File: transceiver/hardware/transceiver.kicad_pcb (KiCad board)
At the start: 2 copper layers, 50 x 50 mm, 62 parts, among them J1 Conn_Coaxial, J2 Conn_Coaxial, J3 Conn_01x04, J4 Conn_01x02, J5 Conn_Coaxial, U2 LR2021, U3 STM32G030K8Tx, U4 MAX-M10S, Y1 32.768KHz, Y3 32MHz 10pF

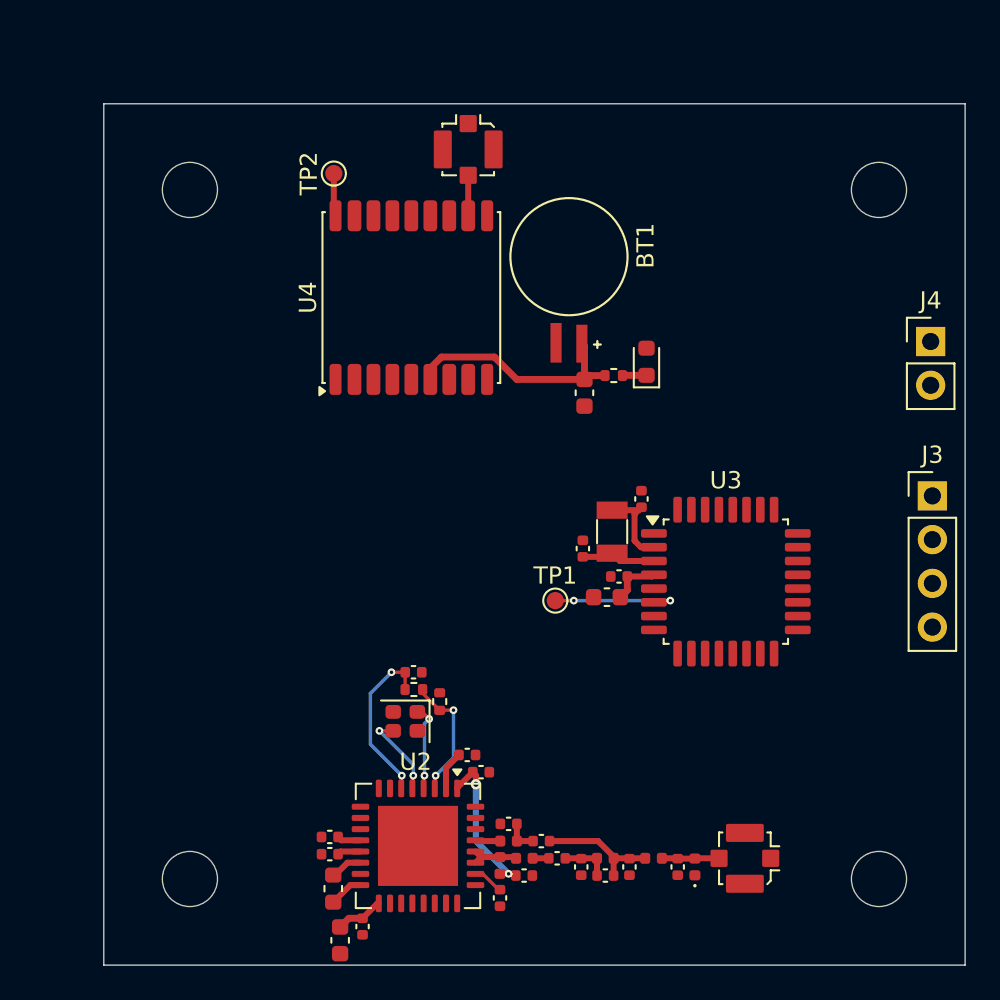
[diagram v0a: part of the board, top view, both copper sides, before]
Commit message: updated board and started frame
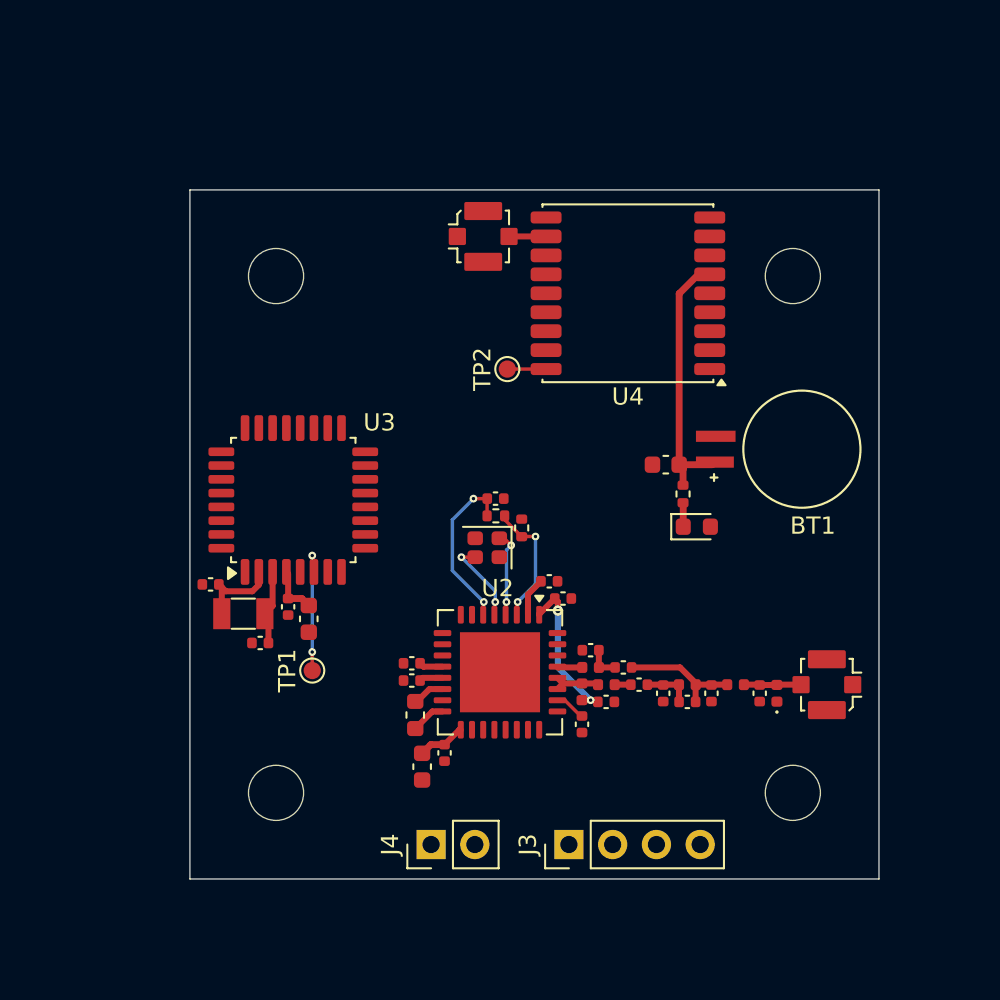
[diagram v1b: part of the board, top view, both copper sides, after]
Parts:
- moved J4 41.2 mm to (129.0, 128.0), turned to 90 degrees
- moved J3 29.2 mm to (137.0, 128.0), turned to 90 degrees
- moved U3 25.6 mm to (121.0, 108.0), turned to 90 degrees
- moved C22 25.5 mm to (116.2, 112.9), turned to 0 degrees
- moved Y1 21.9 mm to (118.1, 114.6), turned to 0 degrees
- moved C23 19.5 mm to (119.1, 116.3), turned to 0 degrees
- moved C18 19.3 mm to (120.7, 114.2), turned to -90 degrees
- moved BT1 17.5 mm to (150.5, 105.0), turned to 180 degrees
- moved C19 17.4 mm to (121.9, 114.9), turned to -90 degrees
- moved TP2 15.2 mm to (133.4, 100.4)
- moved TP1 14.7 mm to (122.1, 117.9), turned to 90 degrees
- moved U4 12.6 mm to (140.4, 96.0), turned to 180 degrees
- moved C14 11.1 mm to (145.3, 119.2)
- moved L11 11.1 mm to (146.7, 118.7)
- moved L8 11.1 mm to (139.2, 118.7)
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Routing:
- net /V_BCKP: track 13.8 -> 15.6 mm
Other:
- board size 50 x 50 mm -> 40 x 40 mm
